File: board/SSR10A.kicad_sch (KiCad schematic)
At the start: 20 parts, among them U1 HLK-PM03, U2 PY32F030K1xTx, U3 PAN2110P0AA, X1 SWD, Y1 16MHz

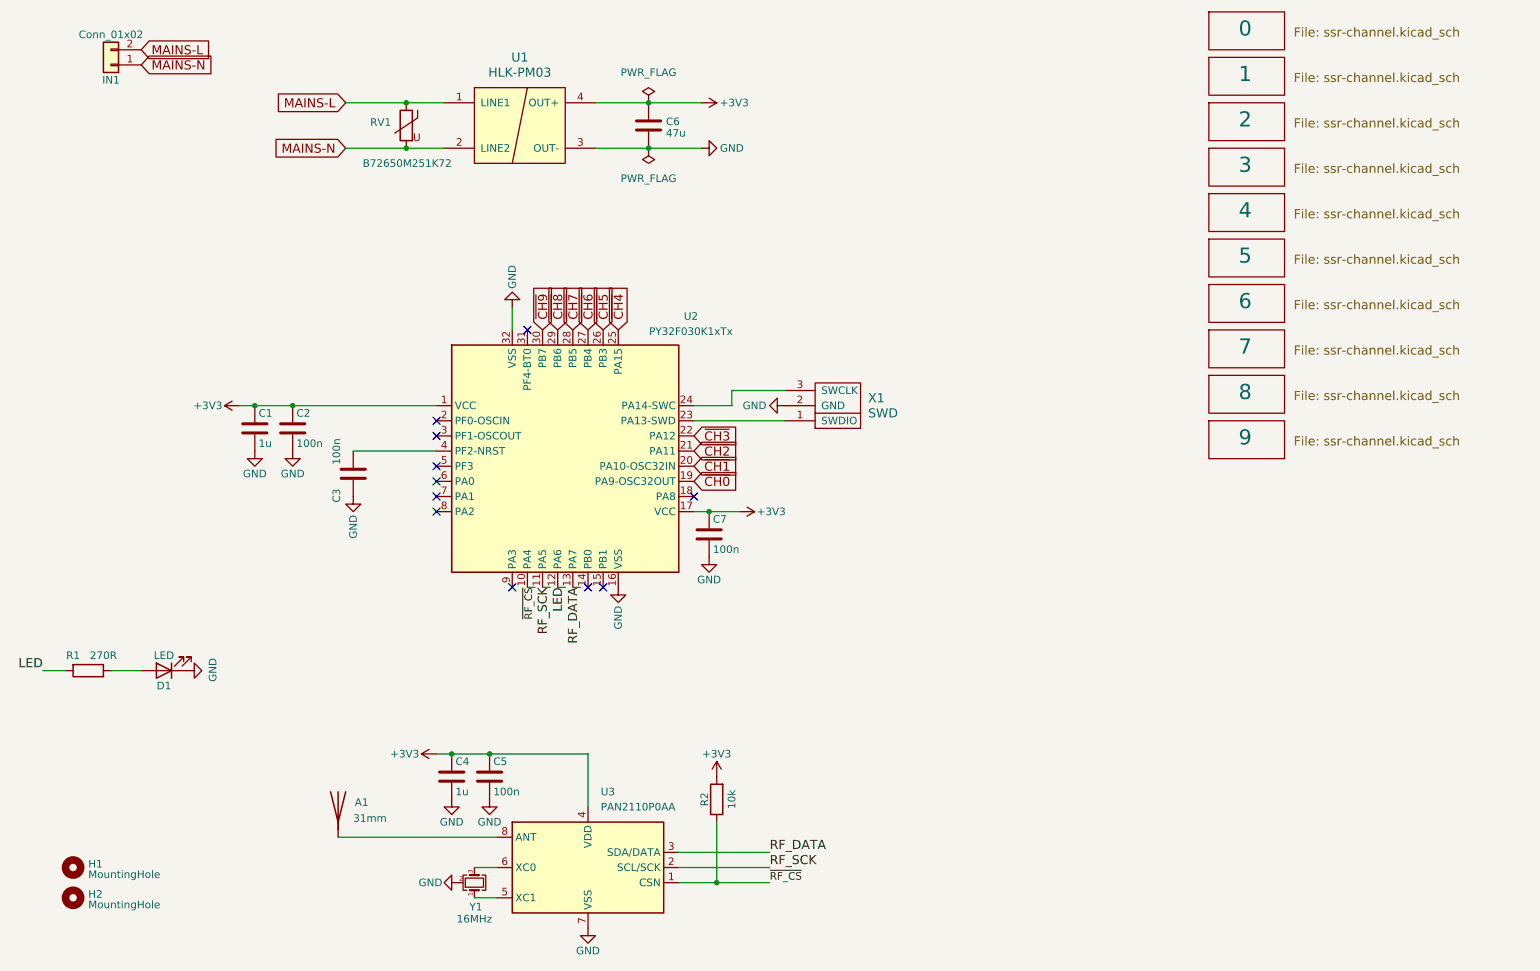
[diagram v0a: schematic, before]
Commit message: Refactor code structure for improved readability and maintainability
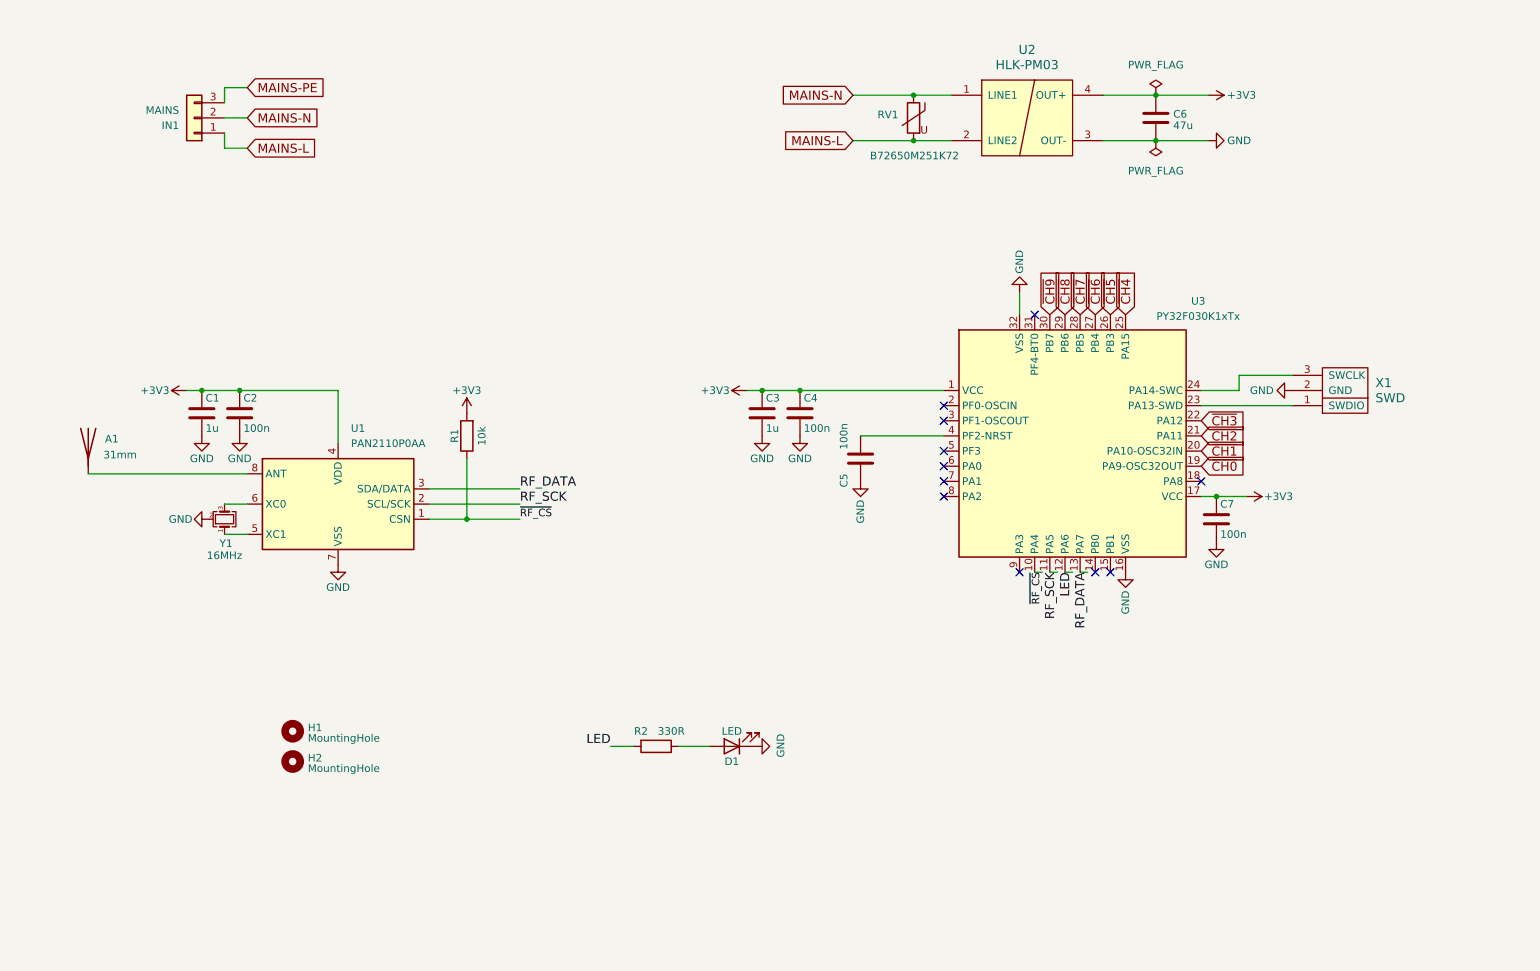
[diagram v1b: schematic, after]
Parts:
- removed IN1: Conn_01x02, Drake:DG235-3.81-02P, symbol Connector_Generic:Conn_01x02
- added IN1: MAINS, Connector_Phoenix_MSTB:PhoenixContact_MSTBA_2,5_3-G_1x03_P5.00mm_Horizontal, symbol Connector_Generic:Conn_01x03
- R2: renamed from R1; value 270R -> 330R
- renumbered C4 to C1, C5 to C2, C1 to C3, C2 to C4, C3 to C5, R2 to R1, U3 to U1, U1 to U2, U2 to U3
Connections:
- net MAINS-L: now also RV1.2, U2.2 (LINE2), IN1.1 (Pin_1); no longer RV1.1, U2.1 (LINE1)
- net MAINS-N: now also RV1.1, U2.1 (LINE1), IN1.2 (Pin_2); no longer RV1.2, U2.2 (LINE2)
- new net MAINS-PE: IN1.3 (Pin_3)
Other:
- removed sheet ssr-channel-${Channel}
- moved on the sheet: A1, C1, C2, C3, C4, C5, C6, C7, D1, H1, H2, R1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
